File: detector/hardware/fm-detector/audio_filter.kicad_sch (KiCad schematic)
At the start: 11 parts, among them J3 U.FL, Q3 BSS138

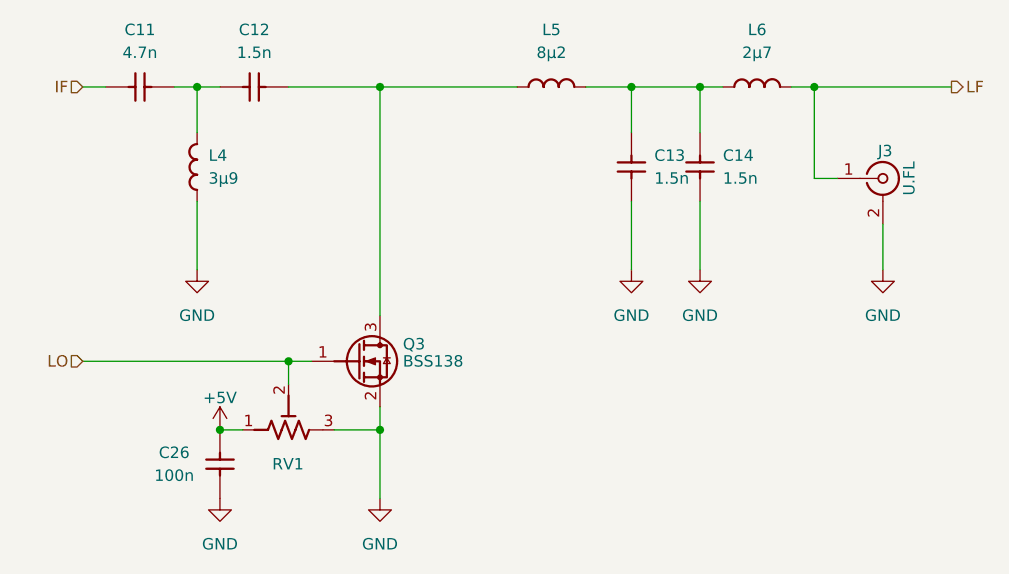
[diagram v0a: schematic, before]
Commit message: pulse detector design
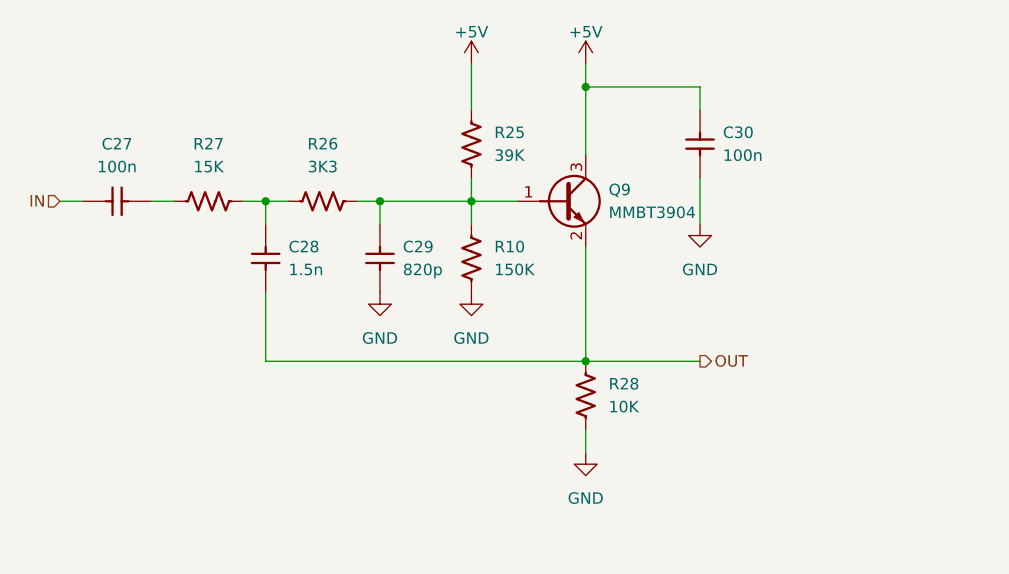
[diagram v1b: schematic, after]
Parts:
- removed C11: 4.7n, g-cap:C_0603_1608Metric, symbol #gplm:cap/CAP-0000-0472
- removed C12, C13, C14: 1.5n, g-cap:C_0603_1608Metric, symbol #gplm:cap/CAP-0000-0152
- removed C26: 100n, g-cap:C_0603_1608Metric, symbol #gplm:cap/CAP-0000-0104
- removed J3: U.FL, g-con:U.FL_Hirose_U.FL-R-SMT-1_Vertical, symbol #gplm:con/CON-0001-0000
- removed L4: 3µ9, g-ind:L_Coilcraft_1008HQ_2520Metric, symbol #gplm:ind/IND-0002-0392
- removed L5: 8µ2, g-ind:L_Coilcraft_1008HQ_2520Metric, symbol #gplm:ind/IND-0002-0822
- removed L6: 2µ7, g-ind:L_Coilcraft_1008HQ_2520Metric, symbol #gplm:ind/IND-0002-0272
- removed Q3: BSS138, g-SOT:SOT-23-3, symbol #gplm:trs/TRS-0001-0000
- removed RV1: 10K, g-rvr:Potentiometer_Bourns_3314J_Vertical, symbol #gplm:rvr/RVR-0000-1002
- added C27, C30: 100n, g-cap:C_0603_1608Metric, symbol #gplm:cap/CAP-0000-0104
- added C28: 1.5n, g-cap:C_0603_1608Metric, symbol #gplm:cap/CAP-0000-0152
- added C29: 820p, g-cap:C_0603_1608Metric, symbol #gplm:cap/CAP-0000-0821
- added Q9: MMBT3904, g-SOT:SOT-23-3, symbol #gplm:trs/TRS-0000-0001
- added R10: 150K, g-res:R_0603_1608Metric, symbol #gplm:res/RES-0000-1503
- added R25: 39K, g-res:R_0603_1608Metric, symbol #gplm:res/RES-0000-3902
- added R26: 3K3, g-res:R_0603_1608Metric, symbol #gplm:res/RES-0000-3301
- added R27: 15K, g-res:R_0603_1608Metric, symbol #gplm:res/RES-0000-1502
- added R28: 10K, g-res:R_0603_1608Metric, symbol #gplm:res/RES-0000-1002
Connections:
- net +5V: now also C30.2, Q9.3 (C), R25.2
- net GND: now also C29.1, C30.1, R10.1, R28.1
- new net: C28.2, R26.1, R27.2
- new net: C29.2, Q9.1 (B), R10.2, R25.1, R26.2
- new net: C27.2, R27.1
- new net IN: C27.1
- new net OUT: C28.1, Q9.2 (E), R28.2
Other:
- title: IF2 Mixer -> Audio filter
